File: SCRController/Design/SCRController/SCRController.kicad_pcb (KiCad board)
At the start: 2 copper layers, 100 x 100 mm, 24 parts, among them Q1 2N2907A, Q2 2N2222A, Q3 2N2222A, Q4 2N2907A, U1 TL084, U2 TL084

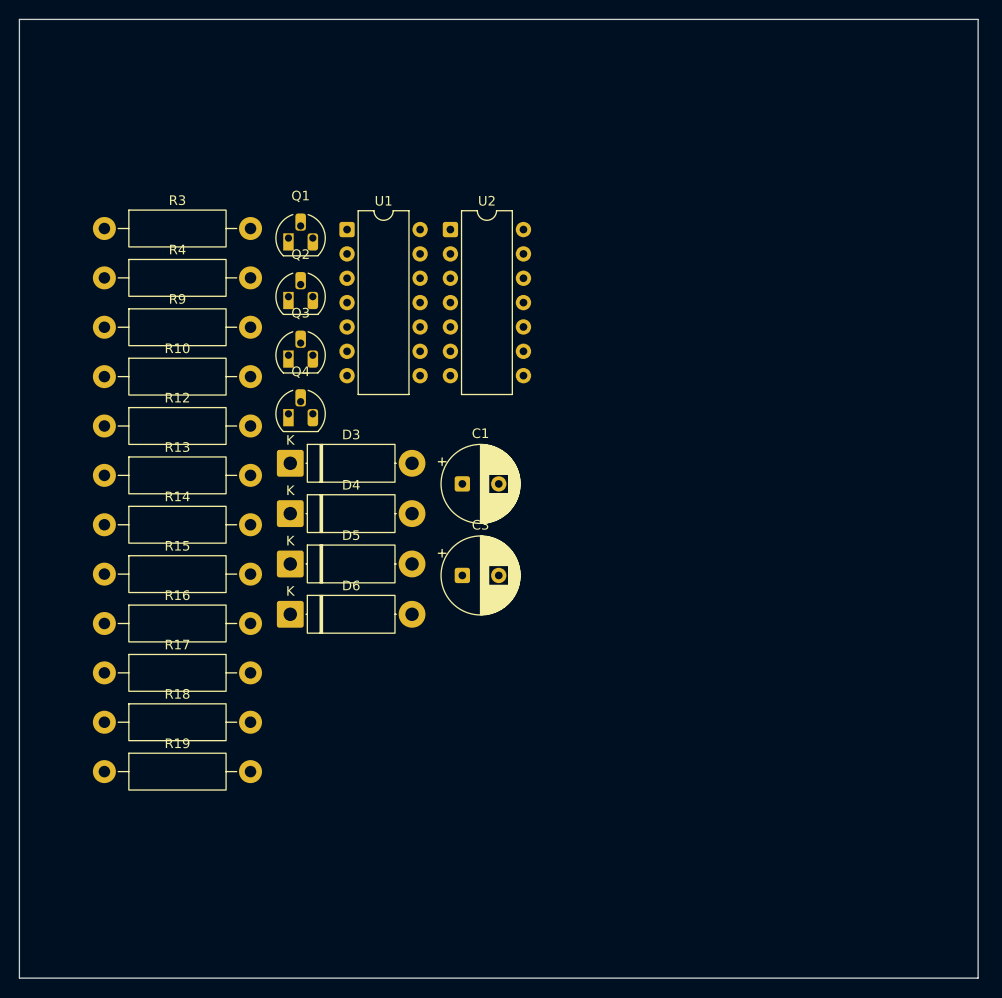
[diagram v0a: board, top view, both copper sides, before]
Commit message: Updated footprints
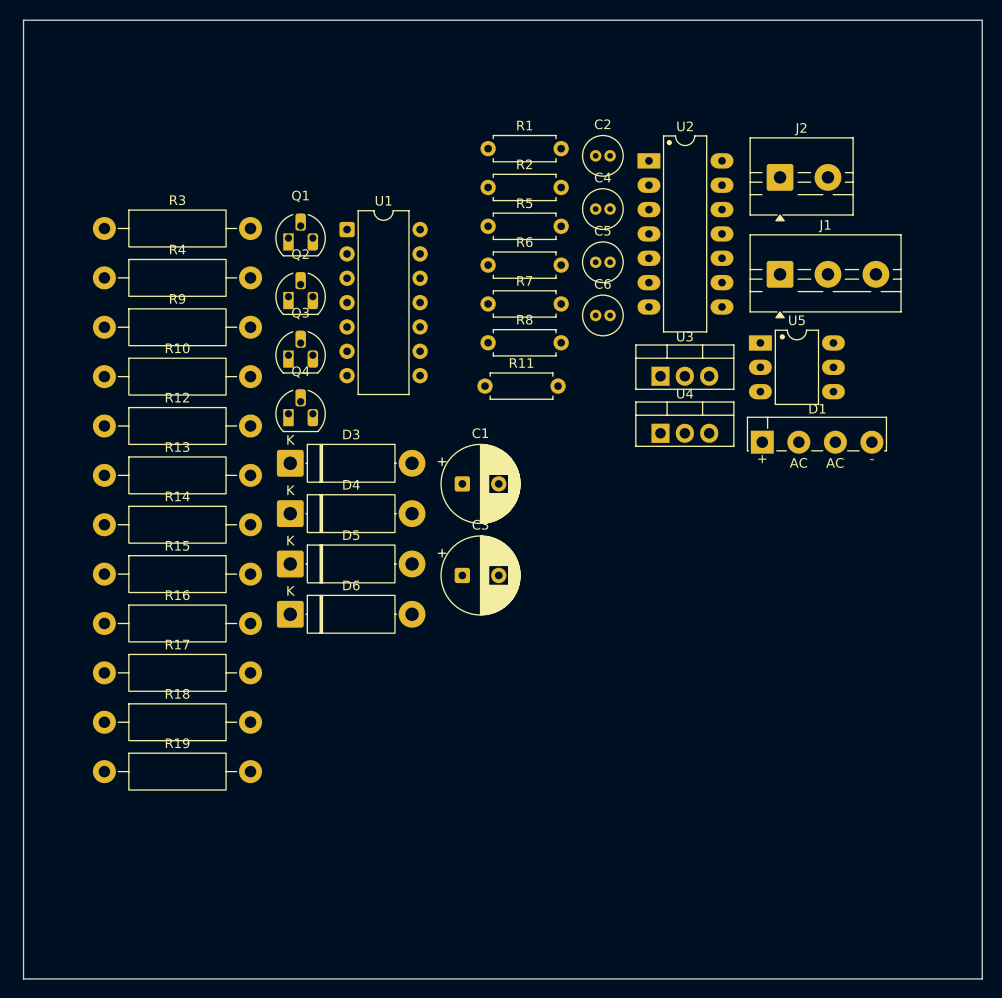
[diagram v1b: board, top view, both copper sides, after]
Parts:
- added C2: C, Capacitor_THT:C_Radial_D4.0mm_H5.0mm_P1.50mm, F.Cu at (160.6, 64.2)
- added C4: C, Capacitor_THT:C_Radial_D4.0mm_H5.0mm_P1.50mm, F.Cu at (160.6, 69.8)
- added C5: C, Capacitor_THT:C_Radial_D4.0mm_H5.0mm_P1.50mm, F.Cu at (160.6, 75.3)
- added C6: C, Capacitor_THT:C_Radial_D4.0mm_H5.0mm_P1.50mm, F.Cu at (160.6, 80.9)
- added D1: KBPC1501W, PCM_Diode_THT_AKL:Diode_Bridge_KBP, F.Cu at (178.0, 94.1)
- added J1: VALT, TerminalBlock:TerminalBlock_MaiXu_MX126-5.0-03P_1x03_P5.00mm, F.Cu at (179.8, 76.6)
- added J2: SAL_TRIAC, TerminalBlock:TerminalBlock_MaiXu_MX126-5.0-02P_1x02_P5.00mm, F.Cu at (179.8, 66.5)
- added R1: 20k, Resistor_THT:R_Axial_DIN0207_L6.3mm_D2.5mm_P7.62mm_Horizontal, F.Cu at (149.4, 63.5)
- added R11: 10k, Resistor_THT:R_Axial_DIN0207_L6.3mm_D2.5mm_P7.62mm_Horizontal, F.Cu at (149.1, 88.2)
- added R2: 20k, Resistor_THT:R_Axial_DIN0207_L6.3mm_D2.5mm_P7.62mm_Horizontal, F.Cu at (149.4, 67.5)
- added R5: 10k, Resistor_THT:R_Axial_DIN0207_L6.3mm_D2.5mm_P7.62mm_Horizontal, F.Cu at (149.4, 71.6)
- added R6: 10k, Resistor_THT:R_Axial_DIN0207_L6.3mm_D2.5mm_P7.62mm_Horizontal, F.Cu at (149.4, 75.6)
- added R7: 220, Resistor_THT:R_Axial_DIN0207_L6.3mm_D2.5mm_P7.62mm_Horizontal, F.Cu at (149.4, 79.7)
- added R8: 1K, Resistor_THT:R_Axial_DIN0207_L6.3mm_D2.5mm_P7.62mm_Horizontal, F.Cu at (149.4, 83.7)
- added U3: LM7815_TO220, Package_TO_SOT_THT:TO-220-3_Vertical, F.Cu at (167.4, 87.2)
- added U4: LM7915_TO220, Package_TO_SOT_THT:TO-220-3_Vertical, F.Cu at (167.4, 93.2)
- added U5: MOC3011M, PCM_Package_DIP_AKL:DIP-6_W7.62mm_LongPads, F.Cu at (177.8, 83.7)
- U2: footprint Package_DIP:CERDIP-14_W7.62mm_SideBrazed -> PCM_Package_DIP_AKL:DIP-14_W7.62mm_LongPads
- moved U2 21.9 mm to (166.2, 64.8)
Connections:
- net Earth renamed DERCENT
- U1 pad 11: (no net) -> VEE
- U1 pad 4: (no net) -> VCC
- U2 pad 1: (no net) -> SUM
- U2 pad 11: unconnected-(U2E-V--Pad11) -> VEE
- U2 pad 2: (no net) -> Net-(U2A--)
- U2 pad 3: (no net) -> Net-(U2A-+)
- U2 pad 4: unconnected-(U2E-V+-Pad4) -> VCC
